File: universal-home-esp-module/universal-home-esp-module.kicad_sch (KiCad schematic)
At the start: 10 parts, among them J1 ES8311 CODEC, J2 LDR MOD, J3 RELAYS, J4 RGB LED, J5 ENV SENSOR, J6 5V PWR, J7 EXT_GPIO, J8 EXT_I2C, U1 ESP32-C3_SUPERMINI_SMD, U2 74HC595

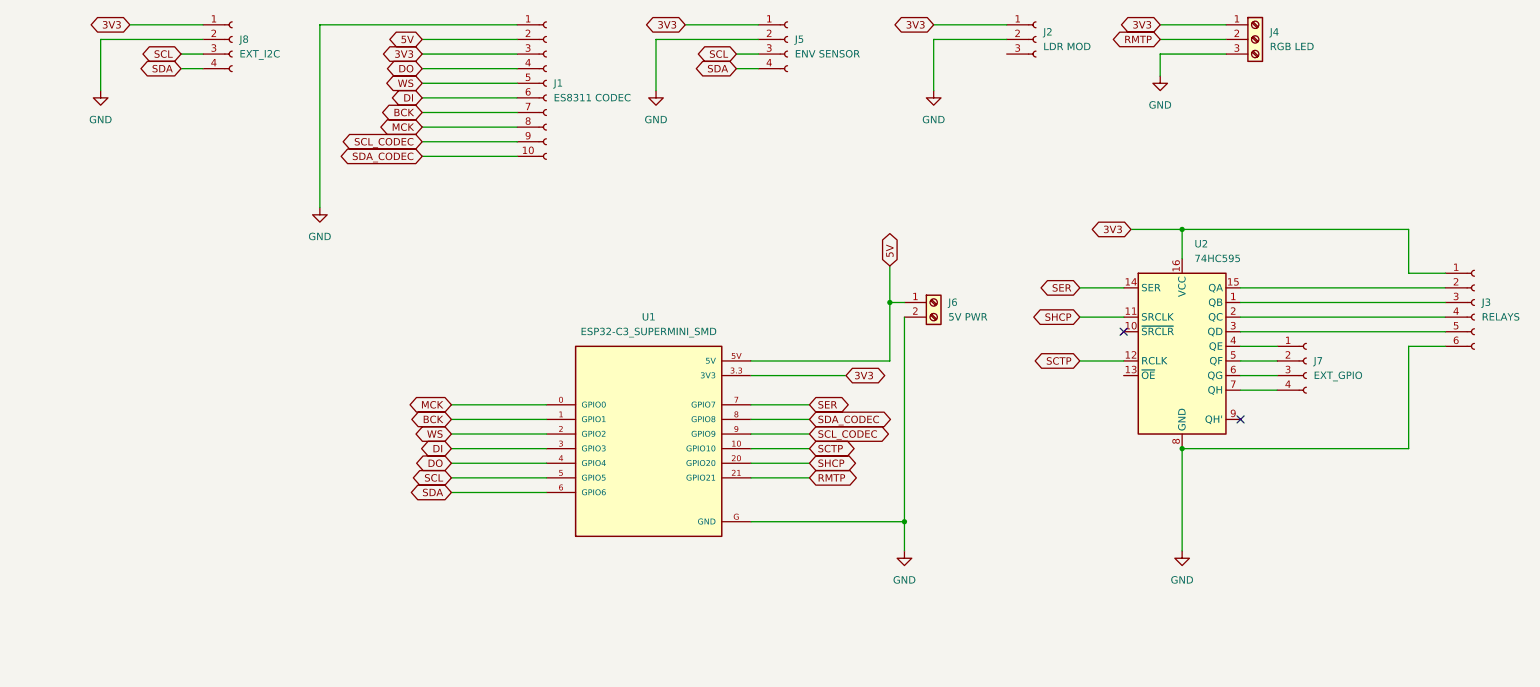
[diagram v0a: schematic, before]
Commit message: first pcb layout
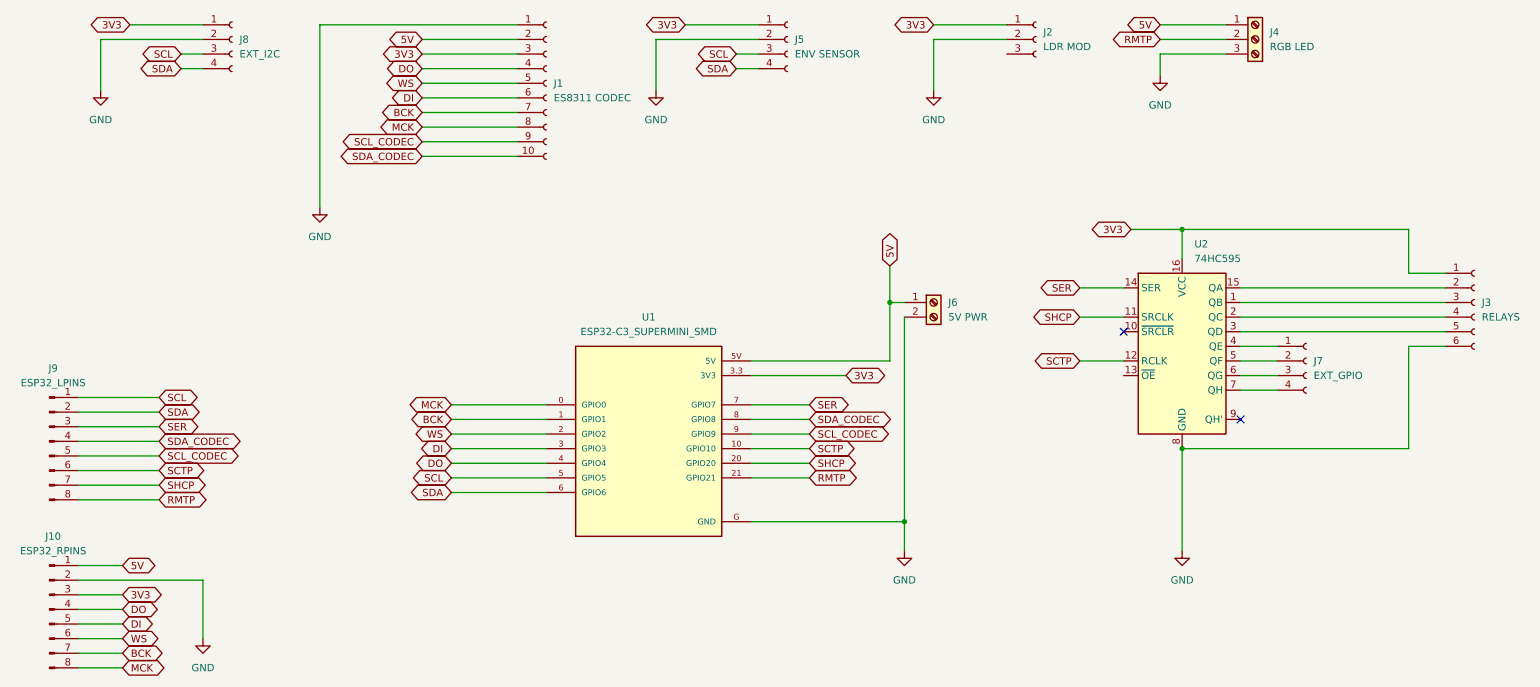
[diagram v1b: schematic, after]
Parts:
- added J10: ESP32_RPINS, Connector_PinSocket_2.54mm:PinSocket_1x08_P2.54mm_Vertical, symbol Connector:Conn_01x08_Pin
- added J9: ESP32_LPINS, Connector_PinSocket_2.54mm:PinSocket_1x08_P2.54mm_Vertical, symbol Connector:Conn_01x08_Pin
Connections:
- net 3V3: now also J10.3 (Pin_3); no longer J4.1 (Pin_1)
- net 5V: now also J4.1 (Pin_1), J10.1 (Pin_1)
- net BCK: now also J10.7 (Pin_7)
- net DI: now also J10.5 (Pin_5)
- net DO: now also J10.4 (Pin_4)
- net GND: now also J10.2 (Pin_2)
- net MCK: now also J10.8 (Pin_8)
- net RMTP: now also J9.8 (Pin_8)
- net SCL: now also J9.1 (Pin_1)
- net SCL_CODEC: now also J9.5 (Pin_5)
- net SCTP: now also J9.6 (Pin_6)
- net SDA: now also J9.2 (Pin_2)
- net SDA_CODEC: now also J9.4 (Pin_4)
- net SER: now also J9.3 (Pin_3)
- net SHCP: now also J9.7 (Pin_7)
- net WS: now also J10.6 (Pin_6)
